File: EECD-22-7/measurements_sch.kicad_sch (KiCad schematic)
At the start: 6 parts, among them J1_I2C_Gamma_Sensor? Conn_01x06_Female, U7 519, U8 DS18B20, U8 MAX485E

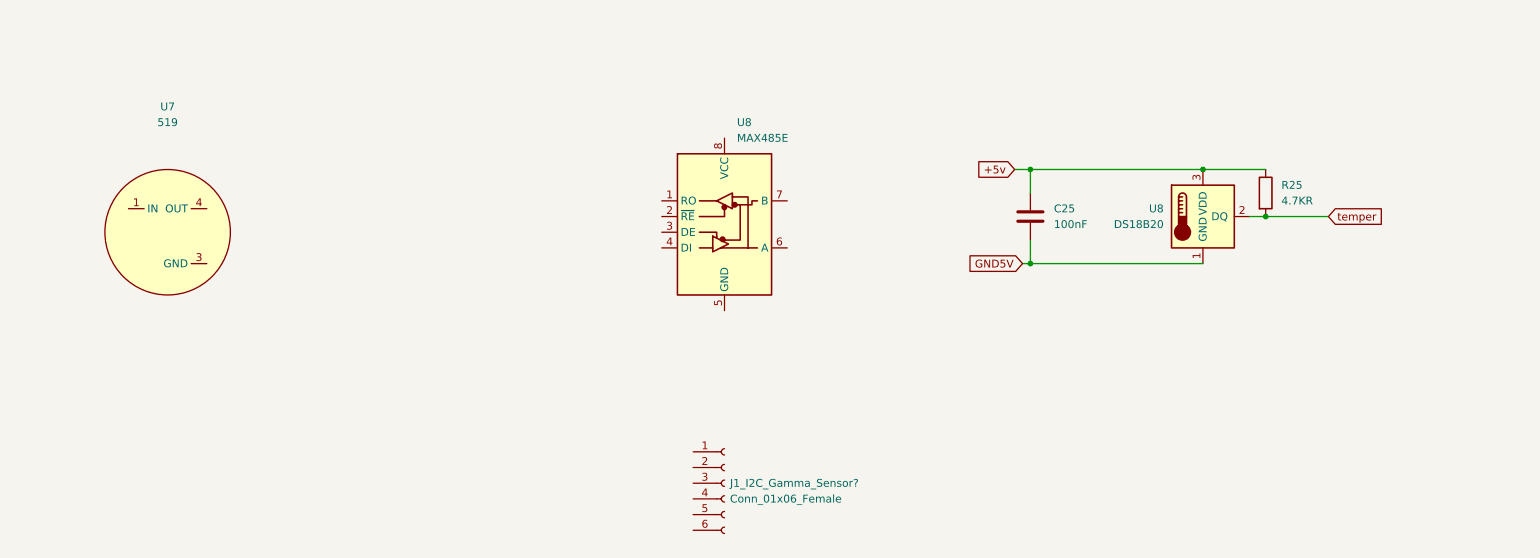
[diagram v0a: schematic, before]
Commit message: Add files via upload
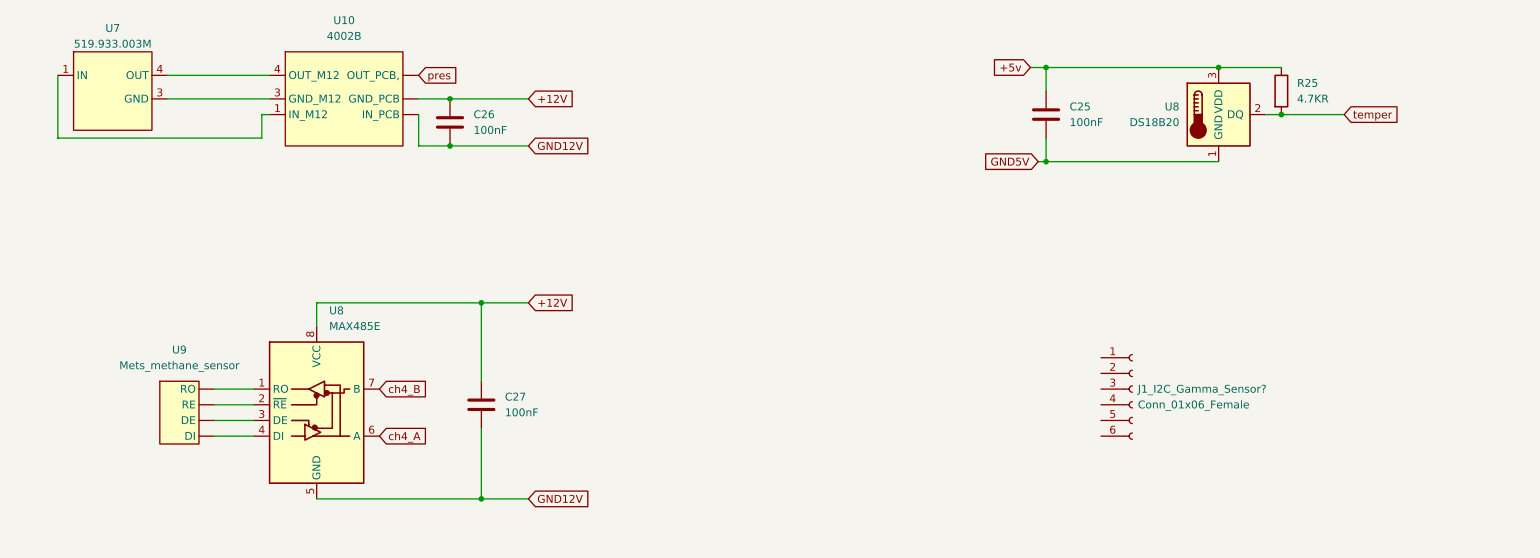
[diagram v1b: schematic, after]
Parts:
- added C26, C27: 100nF, symbol Device:C
- added U10: 4002B, symbol Comparator:4002B
- added U9: Mets_methane_sensor, symbol methane:Mets_methane_sensor
- U7: value 519 -> 519.933.003M
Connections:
- net at U8.1 (RO): now also U9. (RO)
- net at U8.2 (~{RE}): now also U9. (RO)
- net at U8.3 (DE): now also U9. (RO)
- net at U8.4 (DI): now also U9. (RO)
- net GND12V: now reaches U8.5 (GND)
- net GND12V: now also C26.2, C27.2, U10. (OUT_PCB,)
- net ch4_A: now reaches U8.6 (A)
- net ch4_B: now reaches U8.7 (B)
- net +12V: now reaches U8.8 (VCC)
- net +12V: now also C26.1, C27.1, U10. (OUT_PCB,)
- net at U7.1 (IN): now also U10.1 (IN_M12)
- net at U7.3 (GND): now also U10.3 (GND_M12)
- net at U7.4 (OUT): now also U10.4 (OUT_M12)
- new net pres: U10. (OUT_PCB,)
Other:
- moved on the sheet: C25, J1_I2C_Gamma_Sensor?, R25, U7, U8

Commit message: Add files via upload
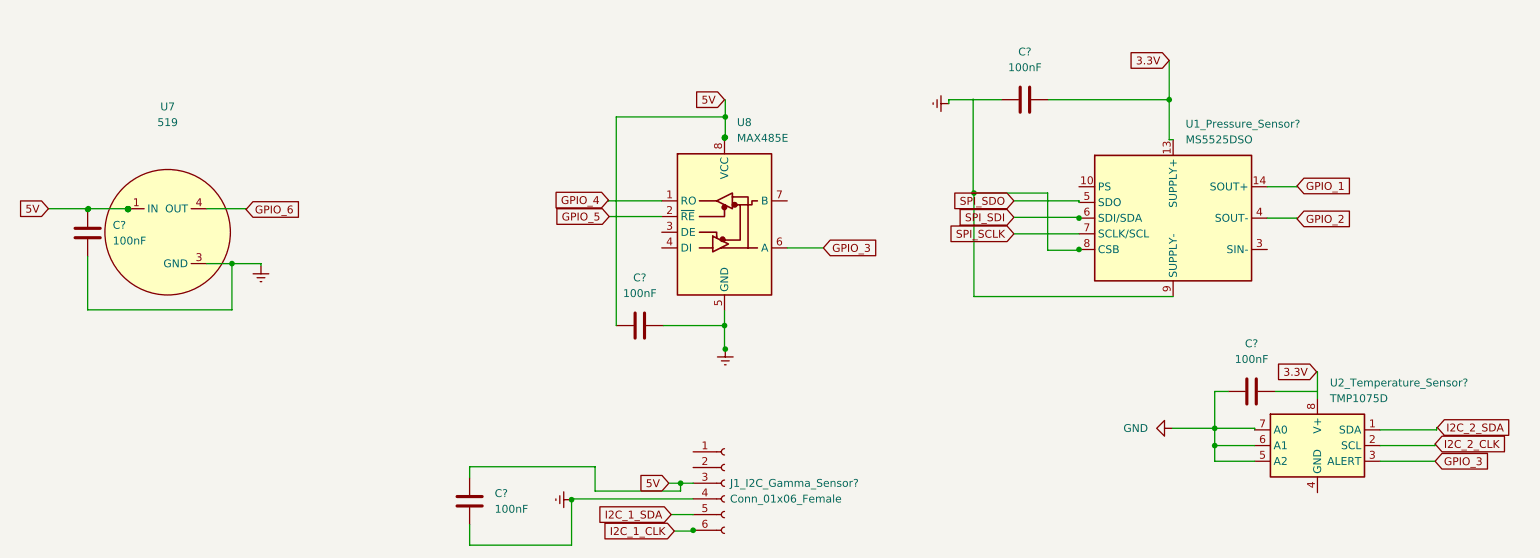
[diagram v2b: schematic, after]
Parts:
- removed C25, C26, C27: 100nF, symbol Device:C
- removed R25: 4.7KR, symbol Device:R
- removed U10: 4002B, symbol Comparator:4002B
- removed U8: DS18B20, Package_TO_SOT_THT:TO-92_Inline, symbol Sensor_Temperature:DS18B20
- removed U9: Mets_methane_sensor, symbol methane:Mets_methane_sensor
- added C? (x5): 100nF, symbol Device:C
- added U1_Pressure_Sensor?: MS5525DSO, symbol Sensor_Pressure:MS5525DSO
- added U2_Temperature_Sensor?: TMP1075D, Package_SO:SO-8_3.9x4.9mm_P1.27mm, symbol Sensor_Temperature:TMP1075D
- U7: value 519.933.003M -> 519
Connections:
- net GND12V is gone; now on net Earth: U8.5 (GND)
- net 5V: now reaches J1_I2C_Gamma_Sensor?.3 (Pin_3)
- net 5V: now also C?.2, C?.2
- net Earth: now reaches J1_I2C_Gamma_Sensor?.4 (Pin_4)
- net Earth: now also U7.3 (GND), C?.1, C?.1, C?.1, C?.2
- net I2C_1_SDA: now reaches J1_I2C_Gamma_Sensor?.5 (Pin_5)
- net I2C_1_CLK: now reaches J1_I2C_Gamma_Sensor?.6 (Pin_6)
- net GPIO_4: now reaches U8.1 (RO)
- net GPIO_5: now reaches U8.2 (~{RE})
- net GPIO_6: now reaches U7.4 (OUT)
- net +12V: no longer names the net of U8.8 (VCC)
- net +12V: now also C?.1
- net ch4_A renamed GPIO_3
- net GPIO_3: now also U2_Temperature_Sensor?.3 (ALERT)
- net ch4_B: no longer names the net of U8.7 (B)
- new net: U1_Pressure_Sensor?.1 (SIN-), U1_Pressure_Sensor?.3 (SIN-)
- new net: U1_Pressure_Sensor?.8 (CSB), U1_Pressure_Sensor?.9 (SUPPLY-)
- new net 3.3V: C?.2, U1_Pressure_Sensor?.11 (SUPPLY+), U1_Pressure_Sensor?.13 (SUPPLY+), U2_Temperature_Sensor?.8 (V+)
- new net GND: C?.1, U2_Temperature_Sensor?.5 (A2), U2_Temperature_Sensor?.6 (A1), U2_Temperature_Sensor?.7 (A0)
- new net GPIO_1: U1_Pressure_Sensor?.12 (SOUT+), U1_Pressure_Sensor?.14 (SOUT+)
- new net GPIO_2: U1_Pressure_Sensor?.2 (SOUT-), U1_Pressure_Sensor?.4 (SOUT-)
- new net I2C_2_CLK: U2_Temperature_Sensor?.2 (SCL)
- new net I2C_2_SDA: U2_Temperature_Sensor?.1 (SDA)
- new net SPI_SCLK: U1_Pressure_Sensor?.7 (SCLK/SCL)
- new net SPI_SDI: U1_Pressure_Sensor?.6 (SDI/SDA)
- new net SPI_SDO: U1_Pressure_Sensor?.5 (SDO)
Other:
- moved on the sheet: J1_I2C_Gamma_Sensor?, U7, U8

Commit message: Add files via upload
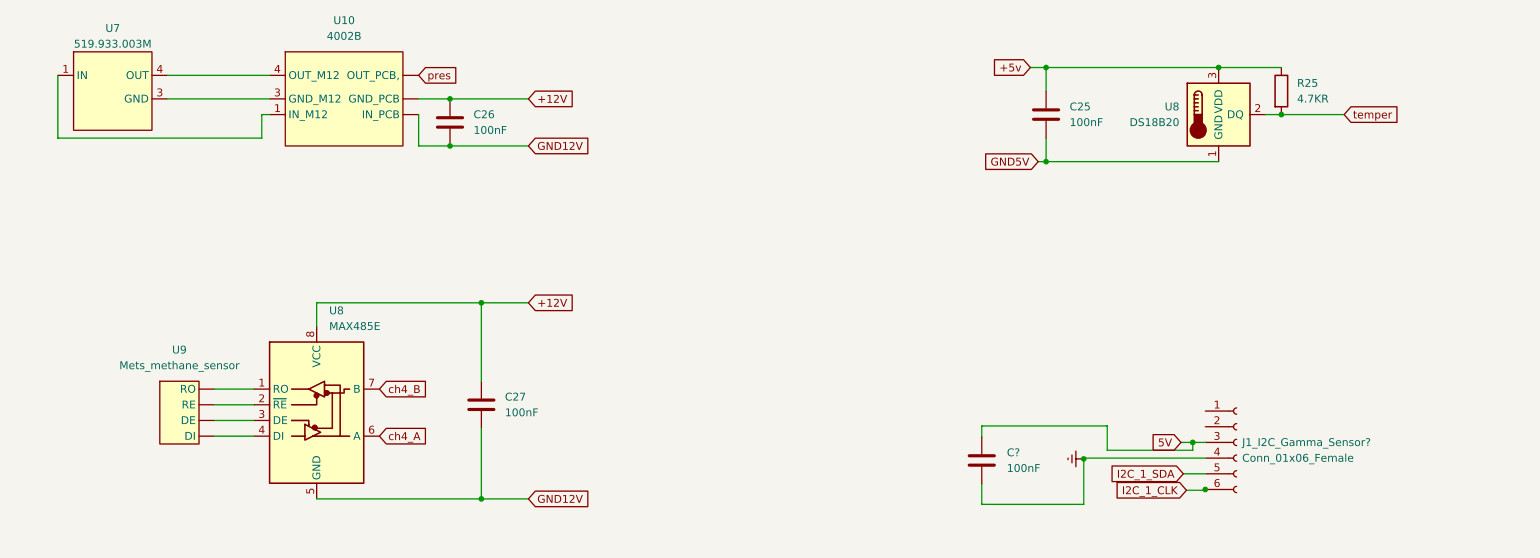
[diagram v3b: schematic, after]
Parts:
- removed C? (x5): 100nF, symbol Device:C
- removed J1_I2C_Gamma_Sensor?: Conn_01x06_Female, symbol Connector:Conn_01x06_Female
- removed U1_Pressure_Sensor?: MS5525DSO, symbol Sensor_Pressure:MS5525DSO
- removed U2_Temperature_Sensor?: TMP1075D, Package_SO:SO-8_3.9x4.9mm_P1.27mm, symbol Sensor_Temperature:TMP1075D
- added C25, C26, C27, C?: 100nF, symbol Device:C
- added J1_I2C_Gamma_Sensor?: Conn_01x06_Female, symbol Connector:Conn_01x06_Female
- added R25: 4.7KR, symbol Device:R
- added U10: 4002B, symbol Comparator:4002B
- added U8: DS18B20, Package_TO_SOT_THT:TO-92_Inline, symbol Sensor_Temperature:DS18B20
- added U9: Mets_methane_sensor, symbol methane:Mets_methane_sensor
- U7: value 519 -> 519.933.003M
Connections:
- net 5V: now also C?.2, J1_I2C_Gamma_Sensor?.3 (Pin_3)
- net Earth: now also C?.1, J1_I2C_Gamma_Sensor?.4 (Pin_4); no longer U7.3 (GND), U8.5 (GND)
- net I2C_1_CLK: now also J1_I2C_Gamma_Sensor?.6 (Pin_6)
- net I2C_1_SDA: now also J1_I2C_Gamma_Sensor?.5 (Pin_5)
- net at U8.3 (DE): now also U9. (RO)
- net at U8.4 (DI): now also U9. (RO)
- net ch4_B: now reaches U8.7 (B)
- net +12V: now reaches U8.8 (VCC)
- net +12V: now also C26.1, C27.1, U10. (OUT_PCB,)
- net at U7.1 (IN): now also U10.1 (IN_M12)
- net GPIO_3 renamed ch4_A
- net GPIO_4: no longer names the net of U8.1 (RO)
- net GPIO_4: now also U9. (RO)
- net GPIO_5: no longer names the net of U8.2 (~{RE})
- net GPIO_5: now also U9. (RO)
- net GPIO_6: no longer names the net of U7.4 (OUT)
- net GPIO_6: now also U10.4 (OUT_M12)
- new net: U10.3 (GND_M12), U7.3 (GND)
- new net +5v: C25.1, R25.1, U8.3 (VDD)
- new net GND12V: C26.2, C27.2, U10. (OUT_PCB,), U8.5 (GND)
- new net GND5V: C25.2, U8.1 (GND)
- new net pres: U10. (OUT_PCB,)
- new net temper: R25.2, U8.2 (DQ)
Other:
- moved on the sheet: U7, U8
